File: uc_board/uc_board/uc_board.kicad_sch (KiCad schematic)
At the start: 5 parts, among them J1 Conn_01x12

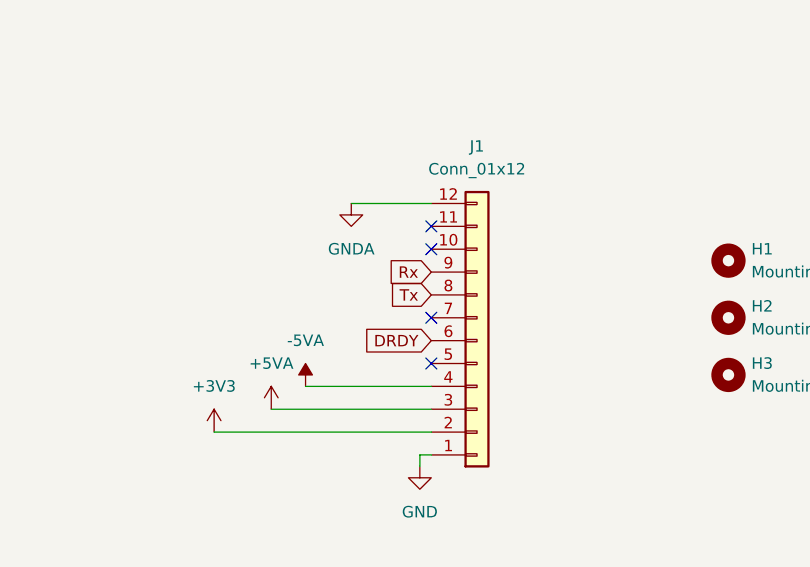
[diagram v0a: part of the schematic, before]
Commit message: update pcb
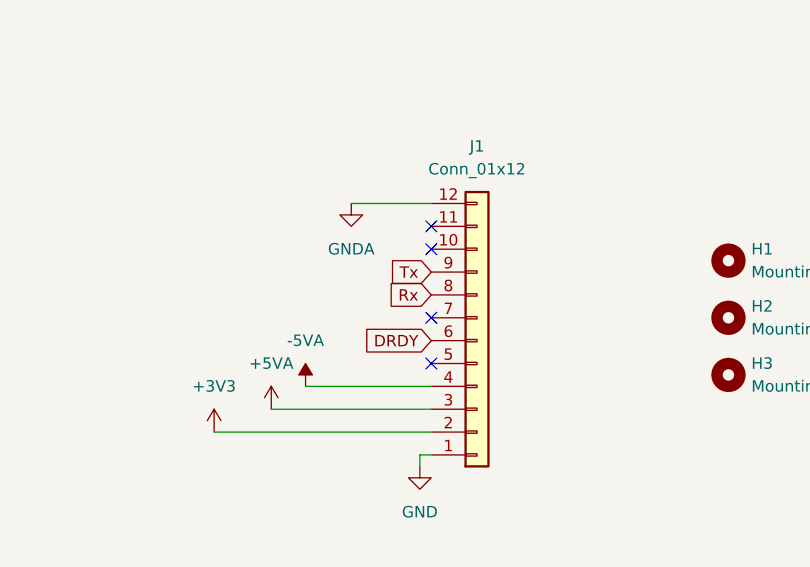
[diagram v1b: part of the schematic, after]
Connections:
- net Rx: now also J1.8 (Pin_8); no longer J1.9 (Pin_9)
- net Tx: now also J1.9 (Pin_9); no longer J1.8 (Pin_8)
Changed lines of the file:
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@@
     )
   )
-  (global_label "Rx" (shape input) (at 212.09 132.08 180) (fields_autoplaced)
+  (global_label "Rx" (shape input) (at 212.09 134.62 180) (fields_autoplaced)
     (effects (font (size 1.27 1.27)) (justify right))
-    (property "Intersheet References" "${INTERSHEET_REFS}" (id 0) (at 207.3788 132.0006 0)
+    (property "Intersheet References" "${INTERSHEET_REFS}" (id 0) (at 207.3788 134.5406 0)
       (effects (font (size 1.27 1.27)) (justify right) hide)
     )
   )
-  (global_label "Tx" (shape input) (at 212.09 134.62 180) (fields_autoplaced)
+  (global_label "Tx" (shape input) (at 212.09 132.08 180) (fields_autoplaced)
     (effects (font (size 1.27 1.27)) (justify right))
-    (property "Intersheet References" "${INTERSHEET_REFS}" (id 0) (at 207.6812 134.5406 0)
+    (property "Intersheet References" "${INTERSHEET_REFS}" (id 0) (at 207.6812 132.0006 0)
       (effects (font (size 1.27 1.27)) (justify right) hide)
     )
